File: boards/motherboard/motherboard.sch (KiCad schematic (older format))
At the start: 36 parts

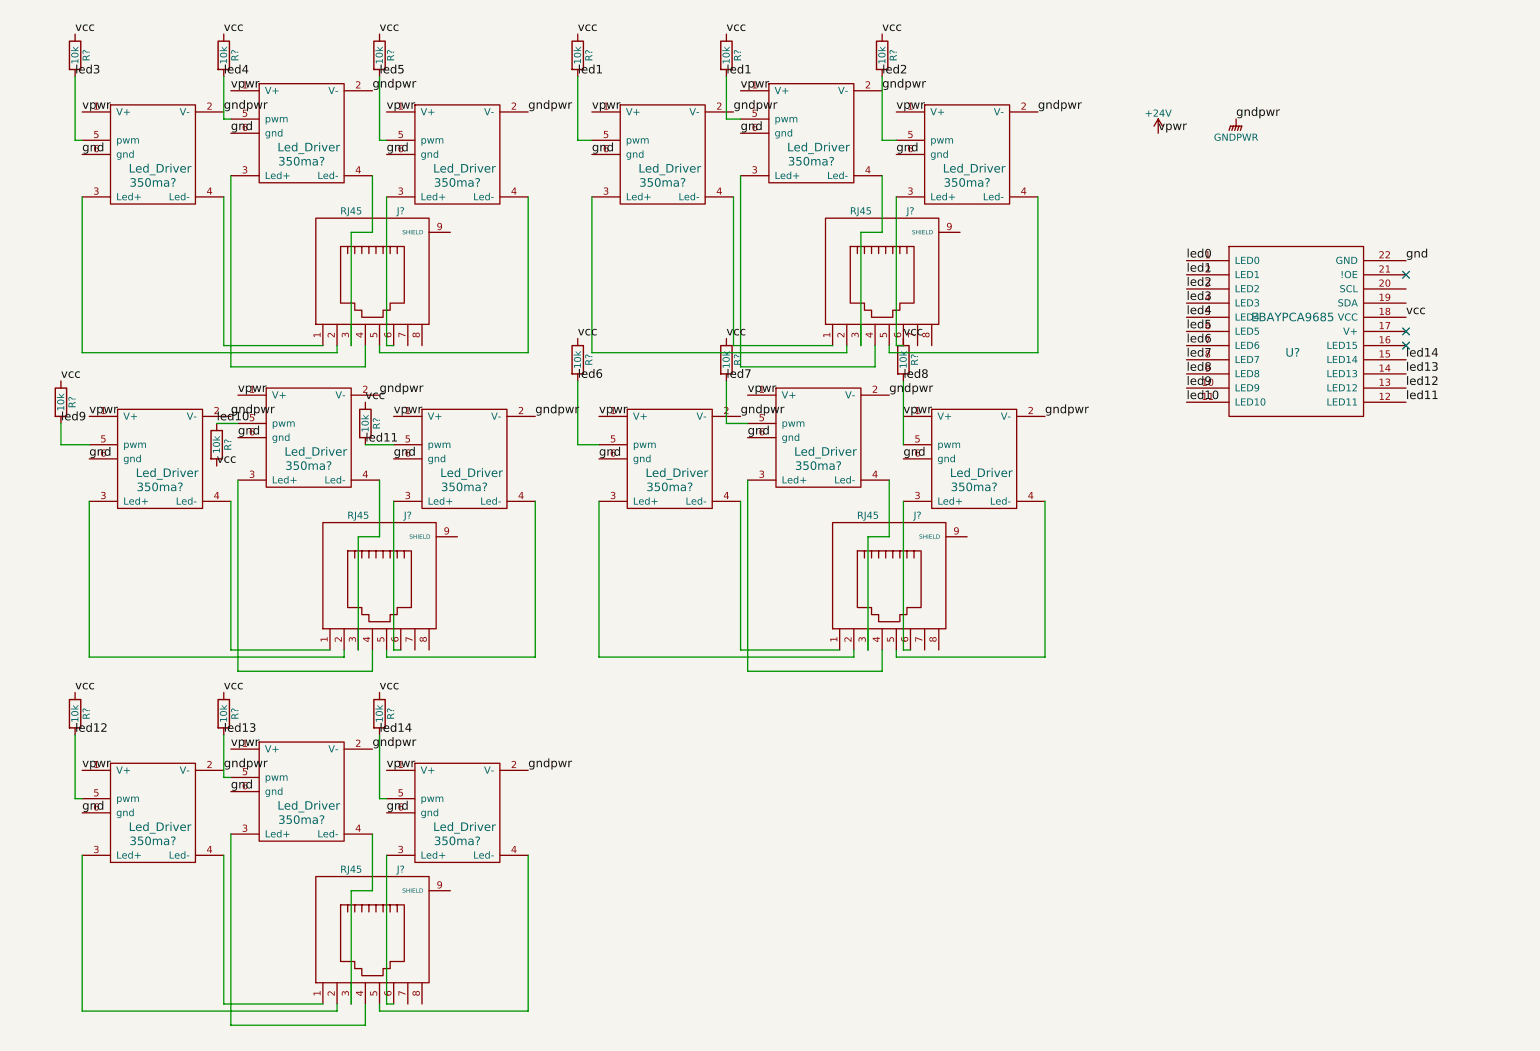
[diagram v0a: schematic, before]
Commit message: updates to mother board
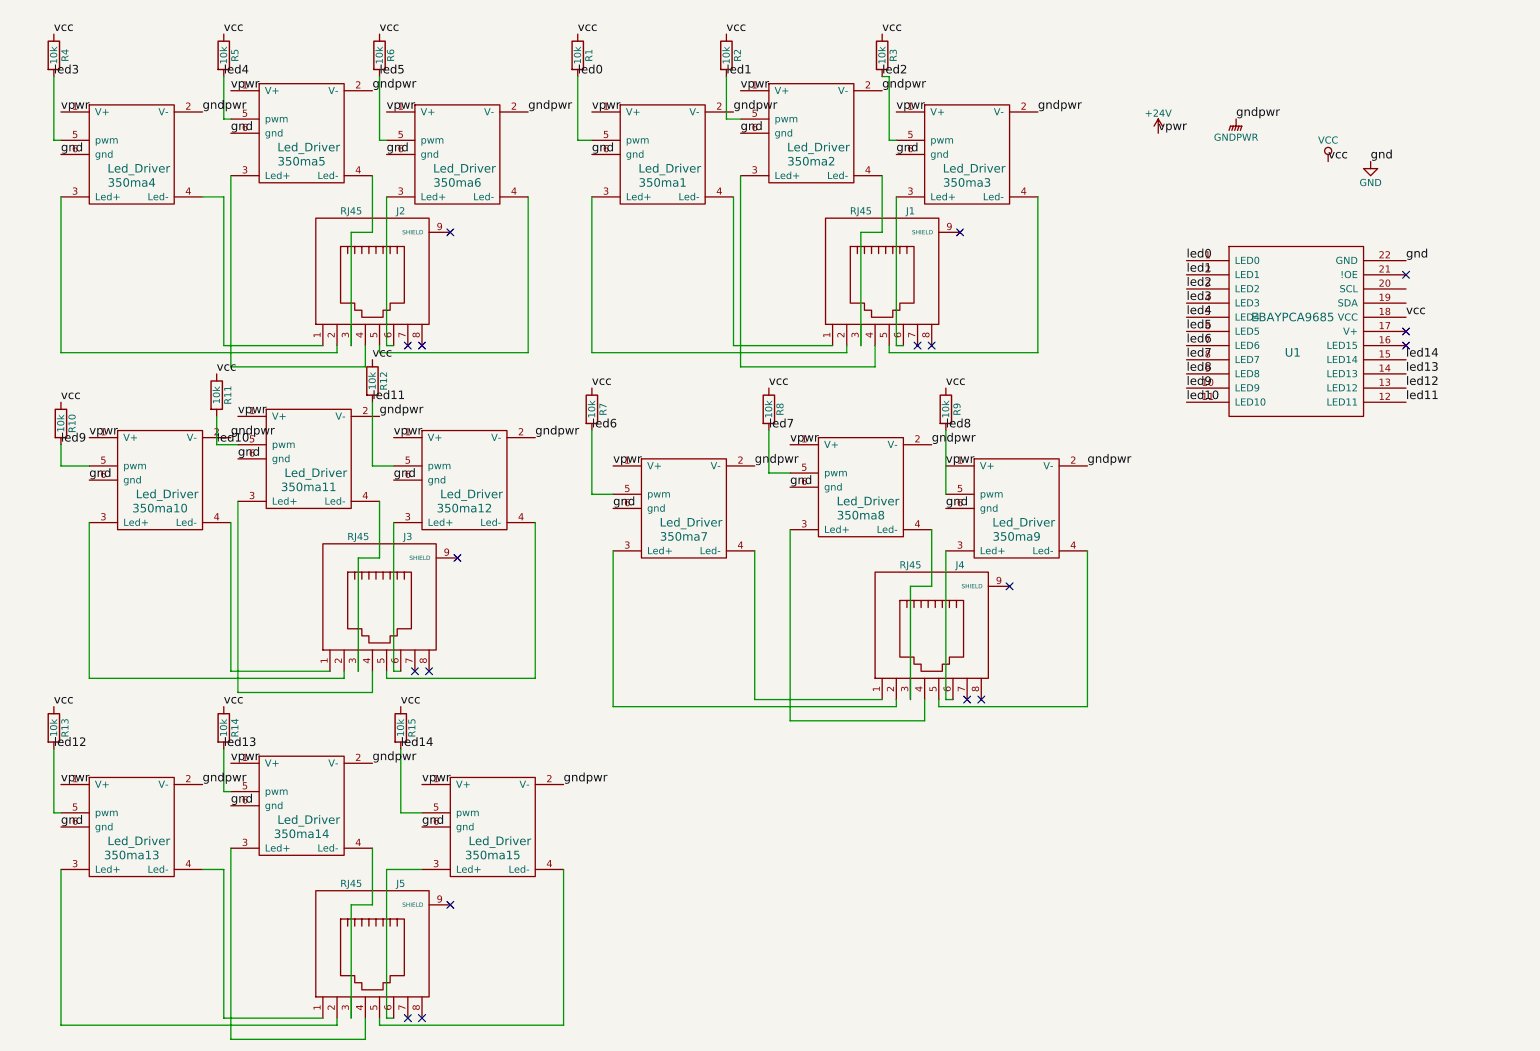
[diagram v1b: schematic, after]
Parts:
- 350ma1, 350ma10, 350ma11, 350ma12, 350ma13, 350ma14, 350ma15, 350ma2, 350ma3, 350ma4, 350ma5, 350ma6, 350ma7, 350ma8, 350ma9: renamed from 350ma?; footprint (none) -> lighting:350ma constant current xl4001
- J1, J2, J3, J4, J5: renamed from J?; footprint (none) -> lighting:RJ45
- R1, R10, R11, R12, R13, R14, R15, R2, R3, R4, R5, R6, R7, R8, R9: renamed from R?; footprint (none) -> Resistors_ThroughHole:Resistor_Horizontal_RM10mm
- U1: renamed from U?; footprint (none) -> lighting:pwm_pca9685
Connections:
- net GNDPWR: no longer 350ma14.5 (pwm), 350ma3.5 (pwm), 350ma5.5 (pwm), R14.2, R3.2, R5.2, U1.14 (LED13), U1.3 (LED2), U1.5 (LED4)
- net VCC: now also R11.1; no longer R11.2
- net led0: now also 350ma1.5 (pwm), R1.2
- net led1: no longer 350ma1.5 (pwm), R1.2
- net led10: now also R11.2; no longer R11.1
- new net led13: 350ma14.5 (pwm), R14.2, U1.14 (LED13)
- new net led2: 350ma3.5 (pwm), R3.2, U1.3 (LED2)
- new net led4: 350ma5.5 (pwm), R5.2, U1.5 (LED4)
- no-connect marks 3 -> 18
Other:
- moved on the sheet: 350ma10, 350ma11, 350ma12, 350ma13, 350ma14, 350ma15, 350ma4, 350ma7, 350ma8, 350ma9, J3, J4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

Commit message: mother board pcb
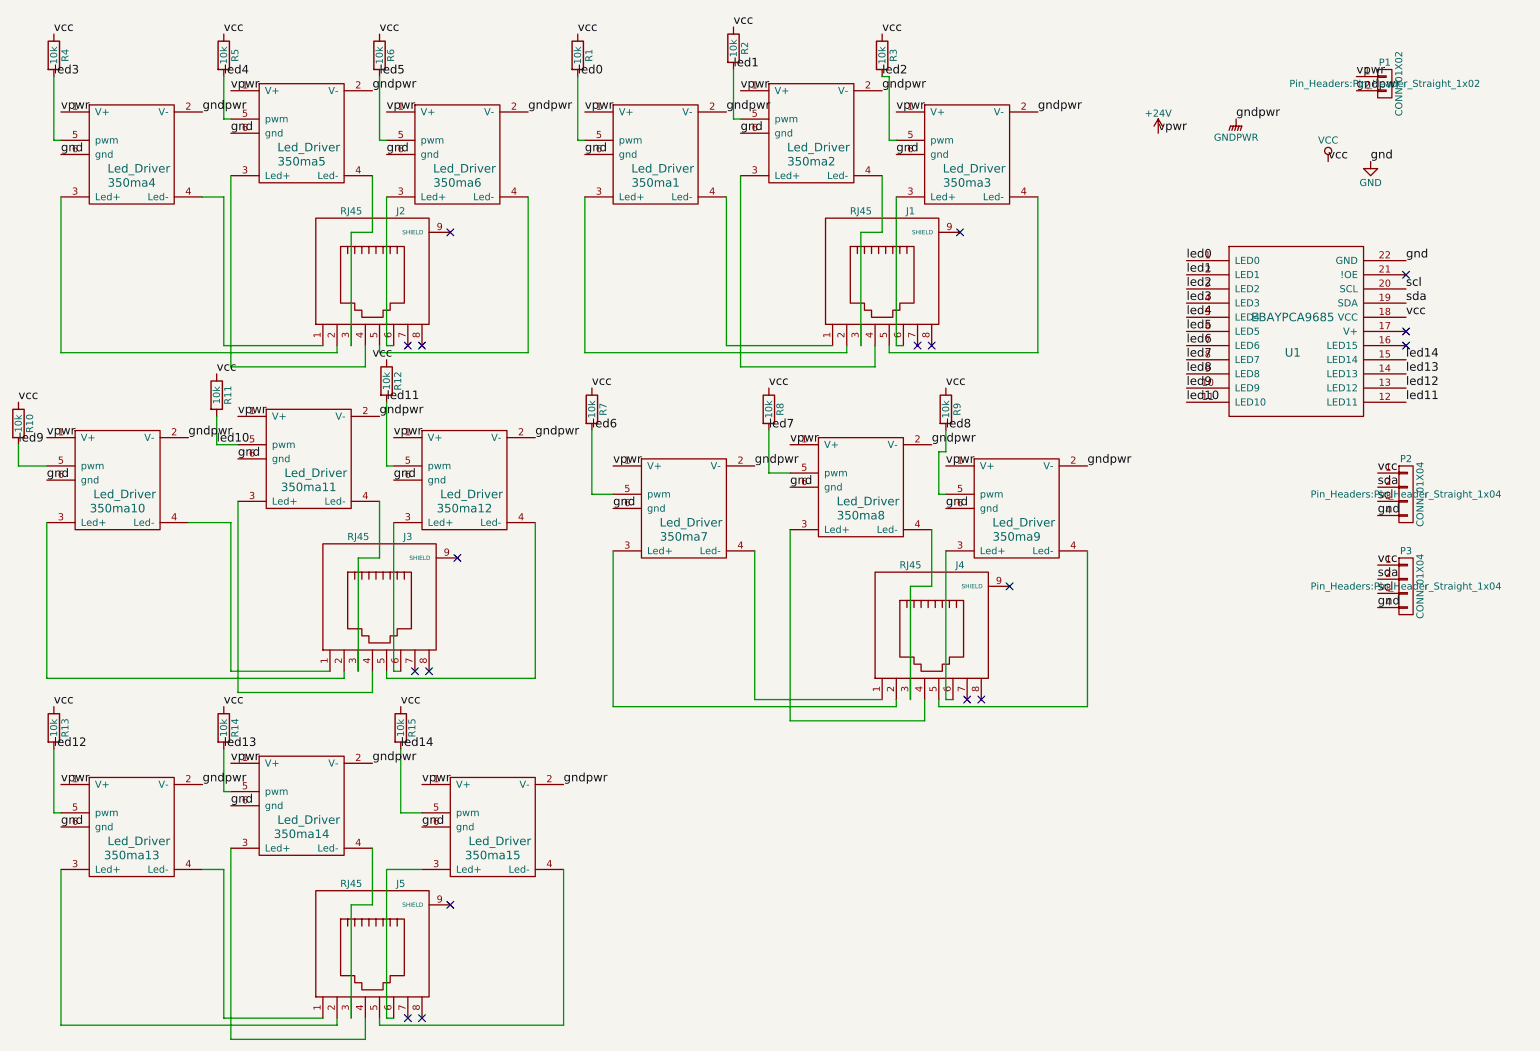
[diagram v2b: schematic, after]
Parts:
- added P1: CONN_01X02, Pin_Headers:Pin_Header_Straight_1x02, symbol CONN_01X02
- added P2, P3: CONN_01X04, Pin_Headers:Pin_Header_Straight_1x04, symbol CONN_01X04
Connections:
- net +24V: now also P1.1 (P1); no longer 350ma9.5 (pwm), R9.2, U1.9 (LED8)
- net GND: now also P2.4 (P4), P3.4 (P4)
- net GNDPWR: now also P1.2 (P2)
- net VCC: now also P2.1 (P1), P3.1 (P1); no longer R12.1
- net sda: now reaches U1.19 (SDA), U1.25 (SDA)
- net sda: now also P2.2 (P2), P3.2 (P2)
- net scl: now reaches U1.20 (SCL), U1.26 (SCL)
- net scl: now also P2.3 (P3), P3.3 (P3)
- new net led8: 350ma9.5 (pwm), R9.2, U1.9 (LED8)
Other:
- moved on the sheet: 350ma1, 350ma10, R10, R12, R2
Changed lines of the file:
@@
 $EndComp
 $Comp
-L +24V #PWR01
+L +24V #PWR1
 U 1 1 5787E774
 P 8600 1350
-F 0 "#PWR01" H 8600 1200 50  0001 C CNN
+F 0 "#PWR1" H 8600 1200 50  0001 C CNN
 F 1 "+24V" H 8600 1490 50  0000 C CNN
 F 2 "" H 8600 1350 50  0000 C CNN
@@
 $EndComp
 $Comp
-L GNDPWR #PWR02
+L GNDPWR #PWR2
 U 1 1 5787E79E
 P 9150 1250
-F 0 "#PWR02" H 9150 1050 50  0001 C CNN
+F 0 "#PWR2" H 9150 1050 50  0001 C CNN
 F 1 "GNDPWR" H 9150 1120 50  0000 C CNN
 F 2 "" H 9150 1200 50  0000 C CNN
@@
 L Led_Driver 350ma1
 U 1 1 5787EC48
-P 5100 1700
-F 0 "350ma1" H 5100 1700 60  0000 C CNN
-F 1 "Led_Driver" H 5150 1800 60  0000 C CNN
-F 2 "lighting:350ma constant current xl4001" H 5100 1700 60  0001 C CNN
-F 3 "" H 5100 1700 60  0000 C CNN
-	1    5100 1700
+P 5050 1700
+F 0 "350ma1" H 5050 1700 60  0000 C CNN
+F 1 "Led_Driver" H 5100 1800 60  0000 C CNN
+F 2 "lighting:350ma constant current xl4001" H 5050 1700 60  0001 C CNN
+F 3 "" H 5050 1700 60  0000 C CNN
+	1    5050 1700
 	1    0    0    -1
 $EndComp
@@
 Text Label 5650 1050 0    60   ~ 0
 vpwr
-Text Label 5600 1200 0    60   ~ 0
-gndpwr
-Text Label 4600 1200 0    60   ~ 0
-vpwr
-Text Label 4600 1500 0    60   ~ 0
+Text Label 5550 1200 0    60   ~ 0
+gndpwr
+Text Label 4550 1200 0    60   ~ 0
+vpwr
+Text Label 4550 1500 0    60   ~ 0
 gnd
 Text Label 5650 1350 0    60   ~ 0
@@
 $EndComp
 $Comp
-L Led_Driver 350ma11
-U 1 1 5787FC55
-P 2600 3850
-F 0 "350ma11" H 2600 3850 60  0000 C CNN
-F 1 "Led_Driver" H 2650 3950 60  0000 C CNN
-F 2 "lighting:350ma constant current xl4001" H 2600 3850 60  0001 C CNN
-F 3 "" H 2600 3850 60  0000 C CNN
-	1    2600 3850
-	1    0    0    -1
-$EndComp
-$Comp
 L Led_Driver 350ma10
 U 1 1 5787FC5B
-P 1550 4000
-F 0 "350ma10" H 1550 4000 60  0000 C CNN
-F 1 "Led_Driver" H 1600 4100 60  0000 C CNN
-F 2 "lighting:350ma constant current xl4001" H 1550 4000 60  0001 C CNN
-F 3 "" H 1550 4000 60  0000 C CNN
-	1    1550 4000
+P 1250 4000
+F 0 "350ma10" H 1250 4000 60  0000 C CNN
+F 1 "Led_Driver" H 1300 4100 60  0000 C CNN
+F 2 "lighting:350ma constant current xl4001" H 1250 4000 60  0001 C CNN
+F 3 "" H 1250 4000 60  0000 C CNN
+	1    1250 4000
 	1    0    0    -1
 $EndComp
@@
 Text Label 2100 3350 0    60   ~ 0
 vpwr
-Text Label 2050 3500 0    60   ~ 0
-gndpwr
-Text Label 1050 3500 0    60   ~ 0
-vpwr
-Text Label 1050 3800 0    60   ~ 0
+Text Label 1750 3500 0    60   ~ 0
+gndpwr
+Text Label 750  3500 0    60   ~ 0
+vpwr
+Text Label 750  3800 0    60   ~ 0
 gnd
 Text Label 2100 3650 0    60   ~ 0
@@
 L R R2
 U 1 1 57881E5D
-P 5550 800
-F 0 "R2" V 5630 800 50  0000 C CNN
-F 1 "10k" V 5550 800 50  0000 C CNN
-F 2 "Resistors_ThroughHole:Resistor_Horizontal_RM10mm" V 5480 800 50  0001 C CNN
-F 3 "" H 5550 800 50  0000 C CNN
-	1    5550 800
-	1    0    0    -1
-$EndComp
-Text Label 5550 650  0    60   ~ 0
+P 5600 750
+F 0 "R2" V 5680 750 50  0000 C CNN
+F 1 "10k" V 5600 750 50  0000 C CNN
+F 2 "Resistors_ThroughHole:Resistor_Horizontal_RM10mm" V 5530 750 50  0001 C CNN
+F 3 "" H 5600 750 50  0000 C CNN
+	1    5600 750
+	1    0    0    -1
+$EndComp
+Text Label 5600 600  0    60   ~ 0
 vcc
 $Comp
@@
 L R R12
 U 1 1 5788238C
-P 3050 3100
-F 0 "R12" V 3130 3100 50  0000 C CNN
-F 1 "10k" V 3050 3100 50  0000 C CNN
-F 2 "Resistors_ThroughHole:Resistor_Horizontal_RM10mm" V 2980 3100 50  0001 C CNN
-F 3 "" H 3050 3100 50  0000 C CNN
-	1    3050 3100
+P 3150 3100
+F 0 "R12" V 3230 3100 50  0000 C CNN
+F 1 "10k" V 3150 3100 50  0000 C CNN
+F 2 "Resistors_ThroughHole:Resistor_Horizontal_RM10mm" V 3080 3100 50  0001 C CNN
+F 3 "" H 3150 3100 50  0000 C CNN
+	1    3150 3100
 	1    0    0    -1
 $EndComp
@@
 L R R10
 U 1 1 5788239A
-P 850 3400
-F 0 "R10" V 930 3400 50  0000 C CNN
-F 1 "10k" V 850 3400 50  0000 C CNN
-F 2 "Resistors_ThroughHole:Resistor_Horizontal_RM10mm" V 780 3400 50  0001 C CNN
-F 3 "" H 850 3400 50  0000 C CNN
-	1    850  3400
-	1    0    0    -1
-$EndComp
-Text Label 850  3250 0    60   ~ 0
+P 550 3400
+F 0 "R10" V 630 3400 50  0000 C CNN
+F 1 "10k" V 550 3400 50  0000 C CNN
+F 2 "Resistors_ThroughHole:Resistor_Horizontal_RM10mm" V 480 3400 50  0001 C CNN
+F 3 "" H 550 3400 50  0000 C CNN
+	1    550  3400
+	1    0    0    -1
+$EndComp
+Text Label 550  3250 0    60   ~ 0
 vcc
 $Comp
@@
 	2850 5200 2850 5150
 Wire Wire Line
-	1050 5200 2850 5200
-Wire Wire Line
-	1050 4100 1050 5200
+	750  5200 2850 5200
+Wire Wire Line
+	750  4100 750  5200
 Wire Wire Line
 	2050 5150 2750 5150
@@
 	6400 2900 6400 2850
 Wire Wire Line
-	4600 2900 6400 2900
-Wire Wire Line
-	4600 1800 4600 2900
-Wire Wire Line
-	5600 2850 6300 2850
-Wire Wire Line
-	5600 1800 5600 2850
-Wire Wire Line
-	7100 3450 7100 3900
+	4550 2900 6400 2900
+Wire Wire Line
+	5550 2850 6300 2850
 Wire Wire Line
 	5850 3450 5850 3750
@@
 	1950 3550 2100 3550
 Wire Wire Line
-	850  3550 850  3700
-Wire Wire Line
-	850  3700 1050 3700
+	550  3550 550  3700
+Wire Wire Line
+	550  3700 750  3700
 Wire Wire Line
 	3250 5700 3250 6150
@@
 	800  6150 850  6150
 Wire Wire Line
-	5550 950  5550 1250
-Wire Wire Line
-	5550 1250 5650 1250
-Wire Wire Line
 	4500 950  4500 1400
-Wire Wire Line
-	4500 1400 4600 1400
 Wire Wire Line
 	3100 950  3100 1400
@@
 Text Label 4500 950  0    60   ~ 0
 led0
-Text Label 5550 950  0    60   ~ 0
+Text Label 5600 900  0    60   ~ 0
 led1
 Text Label 800  950  0    60   ~ 0
@@
 Text Label 5850 3450 0    60   ~ 0
 led7
-Text Label 850  3550 0    60   ~ 0
+Text Label 550  3550 0    60   ~ 0
 led9
 Text Label 1950 3550 0    60   ~ 0
 led10
-Text Label 3050 3250 0    60   ~ 0
+Text Label 3150 3250 0    60   ~ 0
 led11
 Text Label 800  5700 0    60   ~ 0
@@
 NoConn ~ 10350 2350
 Wire Wire Line
-	3050 3250 3050 3700
-Wire Wire Line
-	3050 3700 3200 3700
-Wire Wire Line
 	1950 3350 1950 3550
 NoConn ~ 7200 2050
@@
 NoConn ~ 3400 7600
 $Comp
-L GND #PWR03
+L GND #PWR4
 U 1 1 57888F25
 P 10100 1550
-F 0 "#PWR03" H 10100 1300 50  0001 C CNN
+F 0 "#PWR4" H 10100 1300 50  0001 C CNN
 F 1 "GND" H 10100 1400 50  0000 C CNN
 F 2 "" H 10100 1550 50  0000 C CNN
@@
 $EndComp
 $Comp
-L VCC #PWR04
+L VCC #PWR3
 U 1 1 57888F81
 P 9800 1550
-F 0 "#PWR04" H 9800 1400 50  0001 C CNN
+F 0 "#PWR3" H 9800 1400 50  0001 C CNN
 F 1 "VCC" H 9800 1700 50  0000 C CNN
 F 2 "" H 9800 1550 50  0000 C CNN
@@
 Wire Wire Line
 	6700 950  6650 950
+Wire Wire Line
+	2050 4100 1750 4100
+$Comp
+L Led_Driver 350ma11
+U 1 1 5787FC55
+P 2600 3850
+F 0 "350ma11" H 2600 3850 60  0000 C CNN
+F 1 "Led_Driver" H 2650 3950 60  0000 C CNN
+F 2 "lighting:350ma constant current xl4001" H 2600 3850 60  0001 C CNN
+F 3 "" H 2600 3850 60  0000 C CNN
+	1    2600 3850
+	1    0    0    -1
+$EndComp
+Wire Wire Line
+	3150 3250 3150 3700
+Wire Wire Line
+	3150 3700 3200 3700
+Wire Wire Line
+	5600 900  5600 1250
+Wire Wire Line
+	5600 1250 5650 1250
+Wire Wire Line
+	4500 1400 4550 1400
+Wire Wire Line
+	5550 1800 5550 2850
+Wire Wire Line
+	4550 1800 4550 2900
+Wire Wire Line
+	7100 3450 7100 3600
+Wire Wire Line
+	7100 3600 7050 3600
+Wire Wire Line
+	7050 3600 7050 3900
+Wire Wire Line
+	7050 3900 7100 3900
+$Comp
+L CONN_01X04 P2
+U 1 1 578839F0
+P 10350 3900
+F 0 "P2" H 10350 4150 50  0000 C CNN
+F 1 "CONN_01X04" V 10450 3900 50  0000 C CNN
+F 2 "Pin_Headers:Pin_Header_Straight_1x04" H 10350 3900 50  0000 C CNN
+F 3 "" H 10350 3900 50  0000 C CNN
+	1    10350 3900
+	1    0    0    -1
+$EndComp
+$Comp
+L CONN_01X04 P3
+U 1 1 57883A8C
+P 10350 4550
+F 0 "P3" H 10350 4800 50  0000 C CNN
+F 1 "CONN_01X04" V 10450 4550 50  0000 C CNN
+F 2 "Pin_Headers:Pin_Header_Straight_1x04" H 10350 4550 50  0000 C CNN
+F 3 "" H 10350 4550 50  0000 C CNN
+	1    10350 4550
+	1    0    0    -1
+$EndComp
+$Comp
+L CONN_01X02 P1
+U 1 1 57883AF1
+P 10200 1000
+F 0 "P1" H 10200 1150 50  0000 C CNN
+F 1 "CONN_01X02" V 10300 1000 50  0000 C CNN
+F 2 "Pin_Headers:Pin_Header_Straight_1x02" H 10200 1000 50  0000 C CNN
+F 3 "" H 10200 1000 50  0000 C CNN
+	1    10200 1000
+	1    0    0    -1
+$EndComp
+Text Label 10000 950  0    60   ~ 0
+vpwr
+Text Label 10000 1050 0    60   ~ 0
+gndpwr
+Text Label 10150 3750 0    60   ~ 0
+vcc
+Text Label 10150 4400 0    60   ~ 0
+vcc
+Text Label 10150 3850 0    60   ~ 0
+sda
+Text Label 10150 4500 0    60   ~ 0
+sda
+Text Label 10350 2550 0    60   ~ 0
+sda
+Text Label 10350 2450 0    60   ~ 0
+scl
+Text Label 10150 3950 0    60   ~ 0
+scl
+Text Label 10150 4600 0    60   ~ 0
+scl
+Text Label 10150 4050 0    60   ~ 0
+gnd
+Text Label 10150 4700 0    60   ~ 0
+gnd
 $EndSCHEMATC

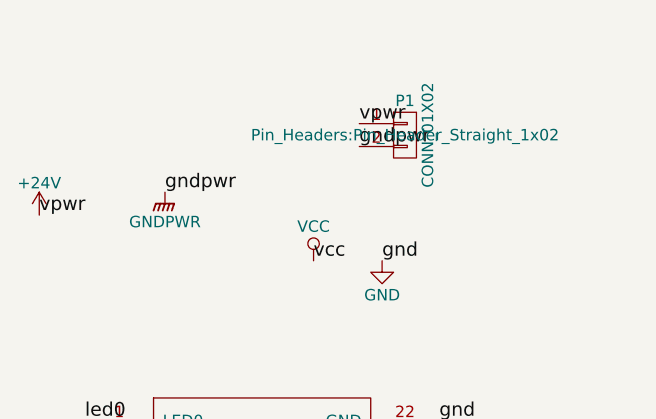
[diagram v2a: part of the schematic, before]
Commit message: before autoroute
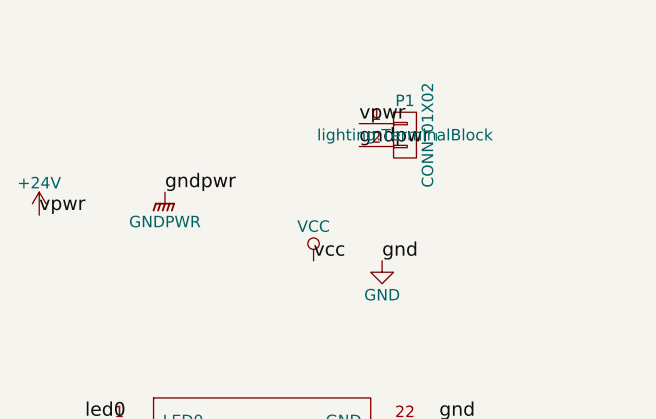
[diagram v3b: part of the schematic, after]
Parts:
- J1, J2, J3, J4, J5: footprint lighting:RJ45 -> Connect:RJ45_8
- P1: footprint Pin_Headers:Pin_Header_Straight_1x02 -> lighting:TerminalBlock
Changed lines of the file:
@@
 F 0 "J1" H 6850 2900 50  0000 C CNN
 F 1 "RJ45" H 6500 2900 50  0000 C CNN
-F 2 "lighting:RJ45" H 6650 2400 50  0001 C CNN
+F 2 "Connect:RJ45_8" H 6650 2400 50  0001 C CNN
 F 3 "" H 6650 2400 50  0000 C CNN
 	1    6650 2400
@@
 F 0 "J4" H 7200 5400 50  0000 C CNN
 F 1 "RJ45" H 6850 5400 50  0000 C CNN
-F 2 "lighting:RJ45" H 7000 4900 50  0001 C CNN
+F 2 "Connect:RJ45_8" H 7000 4900 50  0001 C CNN
 F 3 "" H 7000 4900 50  0000 C CNN
 	1    7000 4900
@@
 F 0 "J2" H 3250 2900 50  0000 C CNN
 F 1 "RJ45" H 2900 2900 50  0000 C CNN
-F 2 "lighting:RJ45" H 3050 2400 50  0001 C CNN
+F 2 "Connect:RJ45_8" H 3050 2400 50  0001 C CNN
 F 3 "" H 3050 2400 50  0000 C CNN
 	1    3050 2400
@@
 F 0 "J3" H 3300 5200 50  0000 C CNN
 F 1 "RJ45" H 2950 5200 50  0000 C CNN
-F 2 "lighting:RJ45" H 3100 4700 50  0001 C CNN
+F 2 "Connect:RJ45_8" H 3100 4700 50  0001 C CNN
 F 3 "" H 3100 4700 50  0000 C CNN
 	1    3100 4700
@@
 F 0 "J5" H 3250 7650 50  0000 C CNN
 F 1 "RJ45" H 2900 7650 50  0000 C CNN
-F 2 "lighting:RJ45" H 3050 7150 50  0001 C CNN
+F 2 "Connect:RJ45_8" H 3050 7150 50  0001 C CNN
 F 3 "" H 3050 7150 50  0000 C CNN
 	1    3050 7150
@@
 F 0 "P1" H 10200 1150 50  0000 C CNN
 F 1 "CONN_01X02" V 10300 1000 50  0000 C CNN
-F 2 "Pin_Headers:Pin_Header_Straight_1x02" H 10200 1000 50  0000 C CNN
+F 2 "lighting:TerminalBlock" H 10200 1000 50  0000 C CNN
 F 3 "" H 10200 1000 50  0000 C CNN
 	1    10200 1000
